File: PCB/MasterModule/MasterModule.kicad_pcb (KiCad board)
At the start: 2 copper layers, 42 x 68.6 mm, 12 parts, among them Con1 Male Connector, Con2 Femail Connector, P1 USB Power, U1 I2C Level Shifter, U2 ESP32

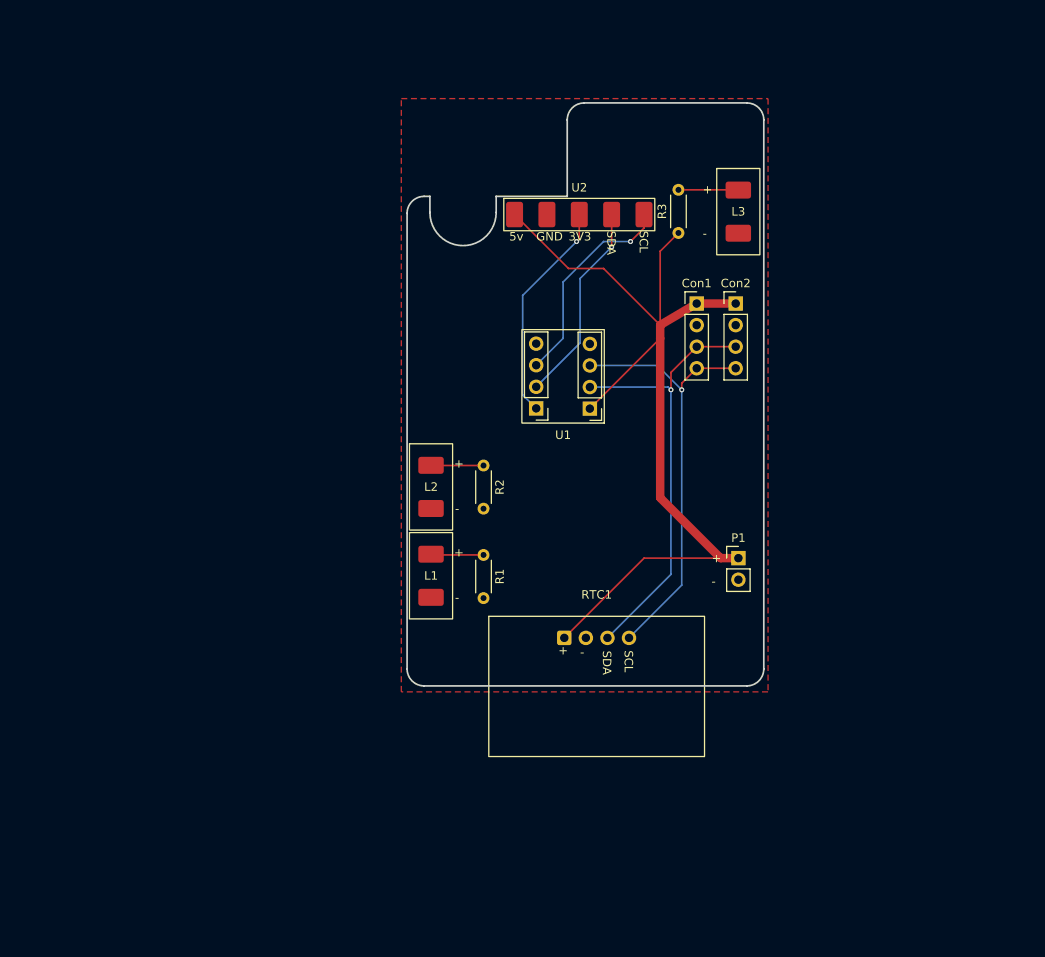
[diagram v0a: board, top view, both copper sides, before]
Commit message: PCB update
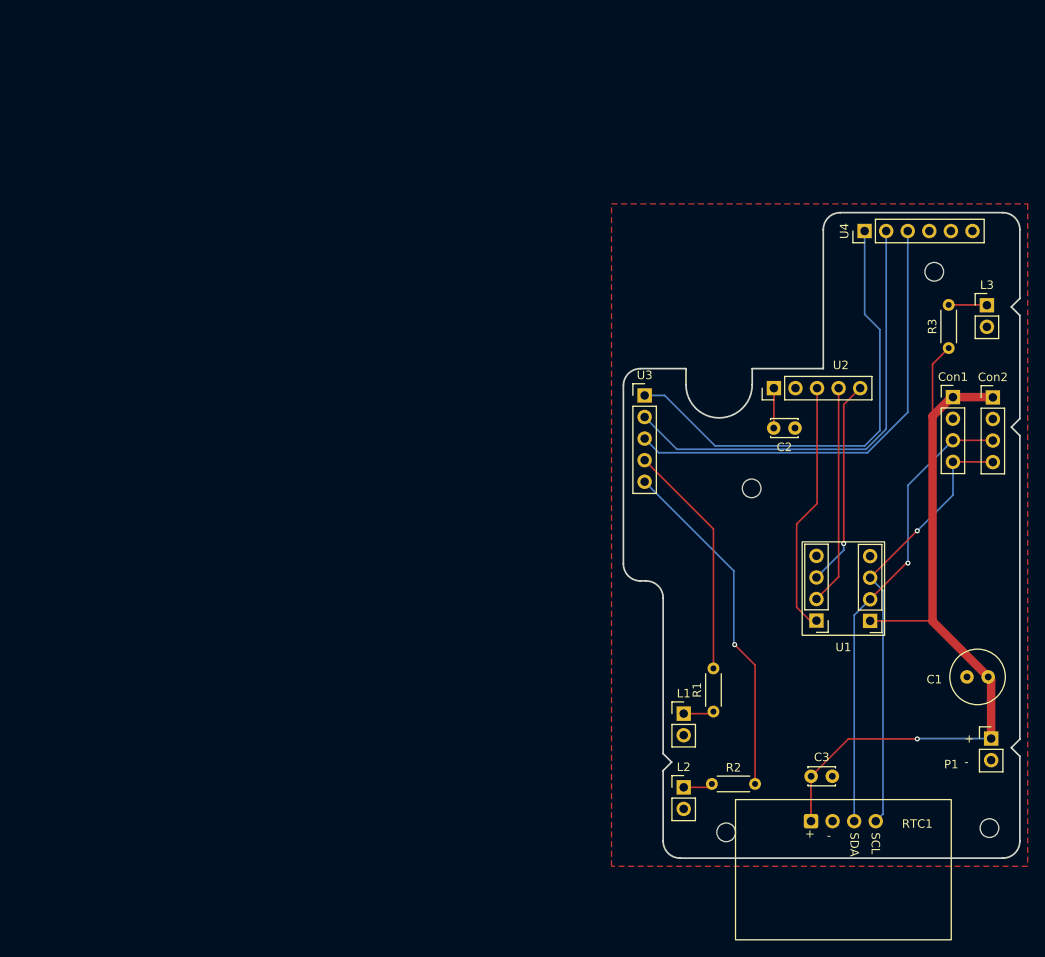
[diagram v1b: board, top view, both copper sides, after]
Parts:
- added C1: 1000uf, Capacitor_THT:C_Radial_D6.3mm_H7.0mm_P2.50mm, F.Cu at (164.3, 122.7)
- added C2: 100nf, Capacitor_THT:C_Disc_D3.0mm_W2.0mm_P2.50mm, F.Cu at (141.6, 93.4)
- added C3: 100nf, Capacitor_THT:C_Disc_D3.0mm_W2.0mm_P2.50mm, F.Cu at (143.5, 134.4)
- added REF**: MountingHole_2.2mm_M2, MountingHole:MountingHole_2.2mm_M2, F.Cu at (164.5, 140.5)
- added REF**: MountingHole_2.2mm_M2, MountingHole:MountingHole_2.2mm_M2, F.Cu at (133.5, 141.0)
- added REF**: MountingHole_2.2mm_M2, MountingHole:MountingHole_2.2mm_M2, F.Cu at (136.5, 100.5)
- added REF**: MountingHole_2.2mm_M2, MountingHole:MountingHole_2.2mm_M2, F.Cu at (158.0, 75.0)
- added U3: ESP32 Signals, Connector_PinHeader_2.54mm:PinHeader_1x05_P2.54mm_Vertical, F.Cu at (123.9, 89.6)
- added U4: Controls, Connector_PinHeader_2.54mm:PinHeader_1x06_P2.54mm_Vertical, F.Cu at (149.8, 70.2)
- L1, L2, L3: footprint 7_Segment_Clock_Footprint_Library:LED_Connection_Footprint -> Connector_PinHeader_2.54mm:PinHeader_1x02_P2.54mm_Vertical
- U2: footprint 7_Segment_Clock_Footprint_Library:ESP32_Connection_Footprint -> Connector_PinHeader_2.54mm:PinHeader_1x05_P2.54mm_Vertical
- moved L2 46.2 mm to (128.5, 135.7)
- moved R2 46.1 mm to (131.8, 135.3), turned to 0 degrees
- moved U1 41.4 mm to (150.4, 116.1)
- moved P1 36.6 mm to (164.7, 130.0)
- moved RTC1 36.2 mm to (147.3, 142.2)
- moved R3 34.6 mm to (159.7, 84.0)
- moved L1 33.9 mm to (128.5, 127.0)
- moved R1 32.8 mm to (132.0, 126.8), turned to 90 degrees
- moved Con2 32.2 mm to (164.9, 89.8)
- moved Con1 32.1 mm to (160.2, 89.8)
- moved L3 31.3 mm to (164.2, 78.9)
- moved U2 30.7 mm to (139.1, 88.7), turned to 90 degrees
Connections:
- R1 pad 2: unconnected-(R1-Pad2) -> Net-(U3-LED1)
- R2 pad 2: unconnected-(R2-Pad2) -> Net-(U3-LED2)
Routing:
- net Net-(U3-Btn1): track 0.00 -> 55.2 mm
- net Net-(U3-SW): track 0.00 -> 55.0 mm
- net Net-(U3-Btn2): track 0.00 -> 54.3 mm
- net Net-(U3-LED2): track 0.00 -> 41.0 mm, vias 0 -> 1
- net Net-(U3-LED1): track 0.00 -> 27.9 mm
- net +5V: track 112.9 -> 98.1 mm, vias 0 -> 1
- net +3V3: track 26.2 -> 29.8 mm, vias 1 -> 0
- net Net-(L2-+): track 6.19 -> 3.49 mm
- net Net-(L1-+): track 6.22 -> 3.60 mm
- net Net-(L3-+): track 7.06 -> 4.52 mm
- net SDA 3V3: track 24.0 -> 25.9 mm, vias 1 -> 0
- net SDA 5V: track 52.9 -> 54.5 mm
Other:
- board size 42 x 68.6 mm -> 46.7 x 76 mm

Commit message: Created (and ordered) the pcb
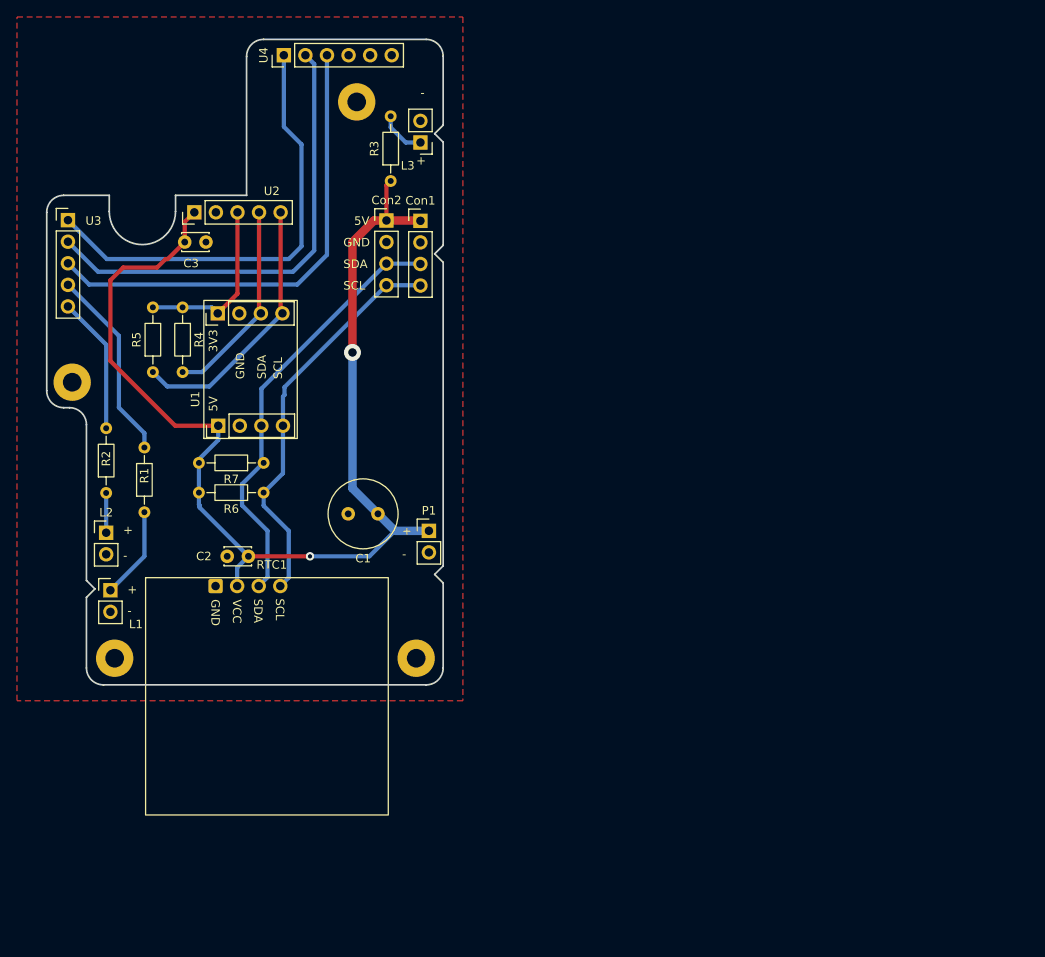
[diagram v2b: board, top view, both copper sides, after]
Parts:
- removed the REF** at (164.5, 140.5)
- removed the REF** at (133.5, 141.0)
- removed the REF** at (136.5, 100.5)
- removed the REF** at (158.0, 75.0)
- added R4: 4k7, Resistor_THT:R_Axial_DIN0204_L3.6mm_D1.6mm_P7.62mm_Horizontal, F.Cu at (69.5, 79.2)
- added R5: 4k7, Resistor_THT:R_Axial_DIN0204_L3.6mm_D1.6mm_P7.62mm_Horizontal, F.Cu at (66.0, 86.8)
- added R6: 4k7, Resistor_THT:R_Axial_DIN0204_L3.6mm_D1.6mm_P7.62mm_Horizontal, F.Cu at (79.0, 101.0)
- added R7: 4k7, Resistor_THT:R_Axial_DIN0204_L3.6mm_D1.6mm_P7.62mm_Horizontal, F.Cu at (79.0, 97.5)
- added REF**: MountingHole_2.2mm_M2_Pad, MountingHole:MountingHole_2.2mm_M2_Pad, F.Cu at (56.5, 88.0)
- added REF**: MountingHole_2.2mm_M2_Pad, MountingHole:MountingHole_2.2mm_M2_Pad, F.Cu at (97.0, 120.5)
- added REF**: MountingHole_2.2mm_M2_Pad, MountingHole:MountingHole_2.2mm_M2_Pad, F.Cu at (61.5, 120.5)
- added REF**: MountingHole_2.2mm_M2_Pad, MountingHole:MountingHole_2.2mm_M2_Pad, F.Cu at (90.0, 55.0)
- C1: footprint Capacitor_THT:C_Radial_D6.3mm_H7.0mm_P2.50mm -> Capacitor_THT:C_Radial_D8.0mm_H11.5mm_P3.50mm
- R1, R2, R3: footprint Resistor_THT:R_Axial_DIN0204_L3.6mm_D1.6mm_P5.08mm_Horizontal -> Resistor_THT:R_Axial_DIN0204_L3.6mm_D1.6mm_P7.62mm_Horizontal
- moved C3 96.9 mm to (69.8, 71.5)
- moved U1 82.3 mm to (73.7, 86.4), turned to 90 degrees
- moved R2 79.1 mm to (60.5, 101.0), turned to 90 degrees
- moved Con2 74.4 mm to (93.5, 69.0)
- moved C1 74.4 mm to (92.5, 103.5)
- moved L2 74.3 mm to (60.5, 105.7)
- moved RTC1 74.2 mm to (77.8, 116.1)
- moved U4 71.4 mm to (81.4, 49.5)
- moved U2 71.3 mm to (70.9, 68.0)
- moved R1 71.0 mm to (65.0, 103.3)
- moved U3 71.0 mm to (56.0, 68.9)
- moved P1 70.6 mm to (98.5, 105.5)
- moved L3 69.4 mm to (97.5, 59.8), turned to 180 degrees
- moved L1 69.0 mm to (61.0, 112.5)
- moved R3 68.6 mm to (94.0, 64.3)
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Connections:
- C2 pad 1: GND -> +5V
- C2 pad 2: +5V -> GND
- RTC1 pad 1: +5V -> GND
- RTC1 pad 2: GND -> +5V
- U1 pad 2: SDA 5V -> GND
- U1 pad 3: SCL 5V -> SDA 5V
- U1 pad 4: GND -> SCL 5V
- U1 pad 6: SDA 3V3 -> GND
- U1 pad 7: SCL 3V3 -> SDA 3V3
- U1 pad 8: GND -> SCL 3V3
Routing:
- net +5V: track 98.1 -> 135.7 mm, vias 1 -> 2
- net Net-(U3-LED2): track 41.0 -> 16.2 mm, vias 1 -> 0
- net +3V3: track 29.8 -> 20.8 mm
- net Net-(L1-+): track 3.60 -> 10.8 mm
- net SCL 3V3: track 24.4 -> 31.5 mm, vias 1 -> 0
- net Net-(U3-LED1): track 27.9 -> 22.9 mm
- net SCL 5V: track 52.1 -> 47.1 mm, vias 1 -> 0
- net SDA 5V: track 54.5 -> 51.3 mm, vias 1 -> 0
- net SDA 3V3: track 25.9 -> 24.1 mm
- net Net-(U3-Btn1): track 55.2 -> 53.4 mm
- net Net-(U3-SW): track 55.0 -> 56.5 mm
- net Net-(L2-+): track 3.49 -> 4.68 mm
- net Net-(L3-+): track 4.52 -> 5.55 mm
- net Net-(U3-Btn2): track 54.3 -> 54.9 mm
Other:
- board text added: "+"
- board text added: "-"
- board text added: "BTN1"
- board text added: "BTN2"
- board text added: "GND"
- board text added: "LED1"
- board text added: "LED2"
- board text added: "SW"
